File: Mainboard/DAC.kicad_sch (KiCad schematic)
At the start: 32 parts, among them IC1 REF102AU_2K5, IC4 DAC8814IBDBT, U2 TL072, U5 TL074, U6 TL074, U7 ADG419BR

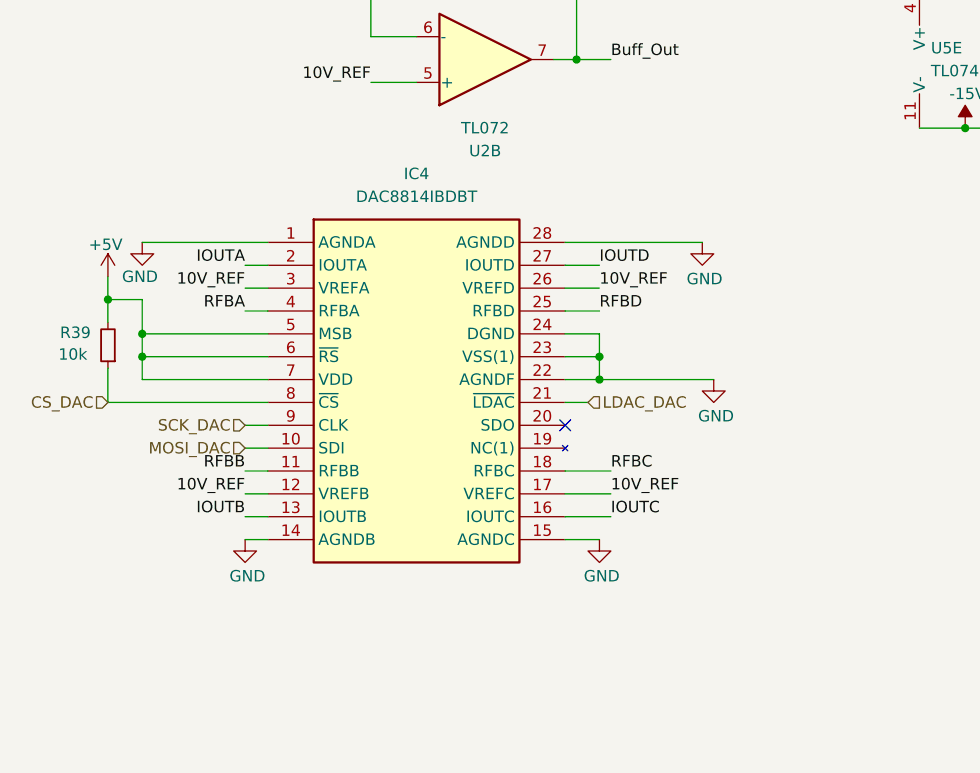
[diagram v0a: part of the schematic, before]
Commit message: Mainboard grind
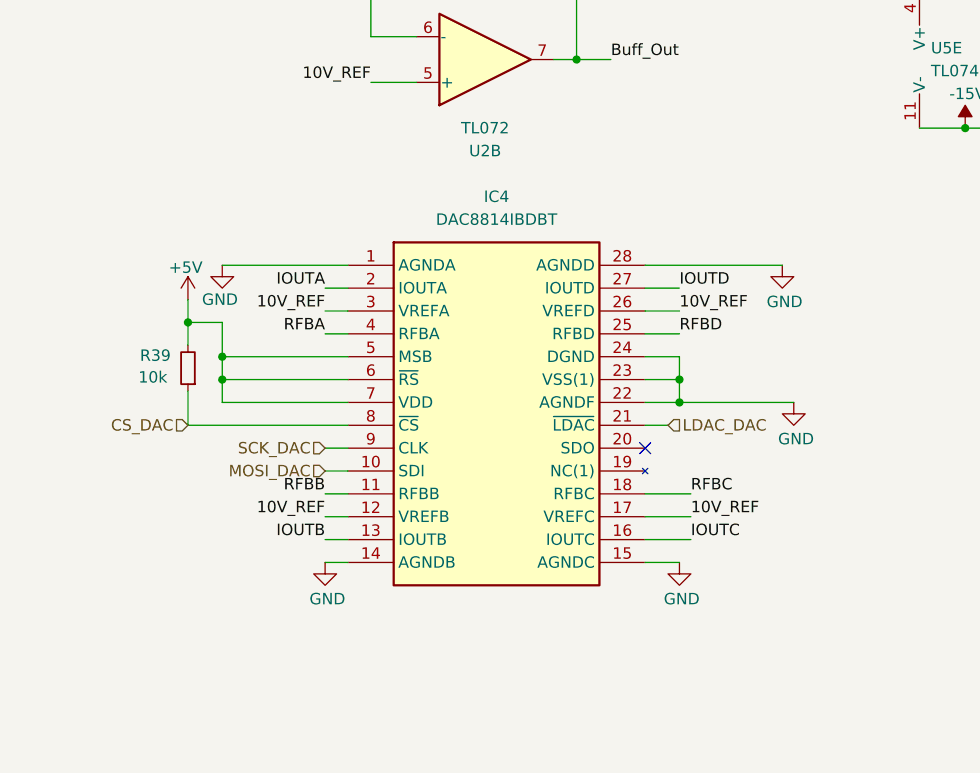
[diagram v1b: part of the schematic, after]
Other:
- moved on the sheet: IC4, R39
